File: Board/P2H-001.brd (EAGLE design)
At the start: 94.9 x 72.4 mm, 29 parts, among them IC1 74LS157N, IC2 LTC485N, IC3 74LS07N, IC4 LTC485N, IC5 TLC5941NT, IC6 TLC5941NT

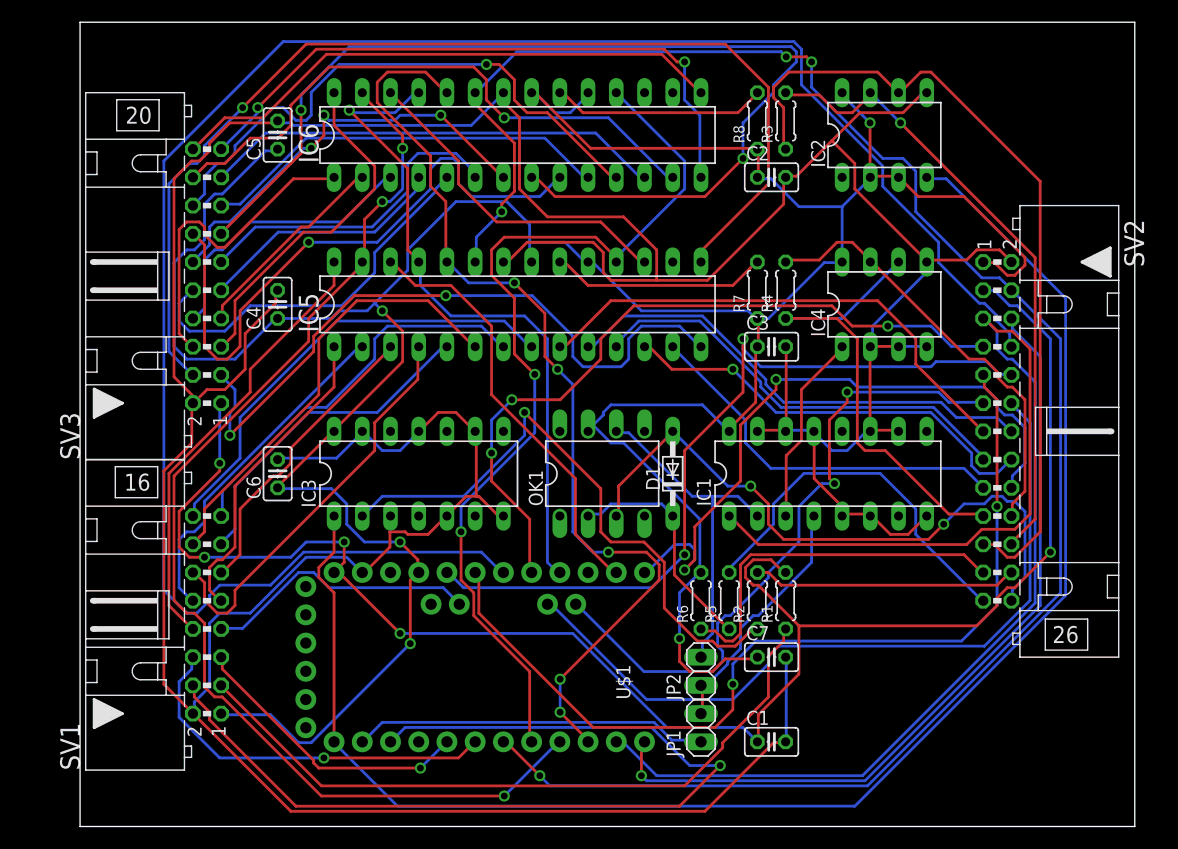
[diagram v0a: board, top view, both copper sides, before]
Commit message: square design.
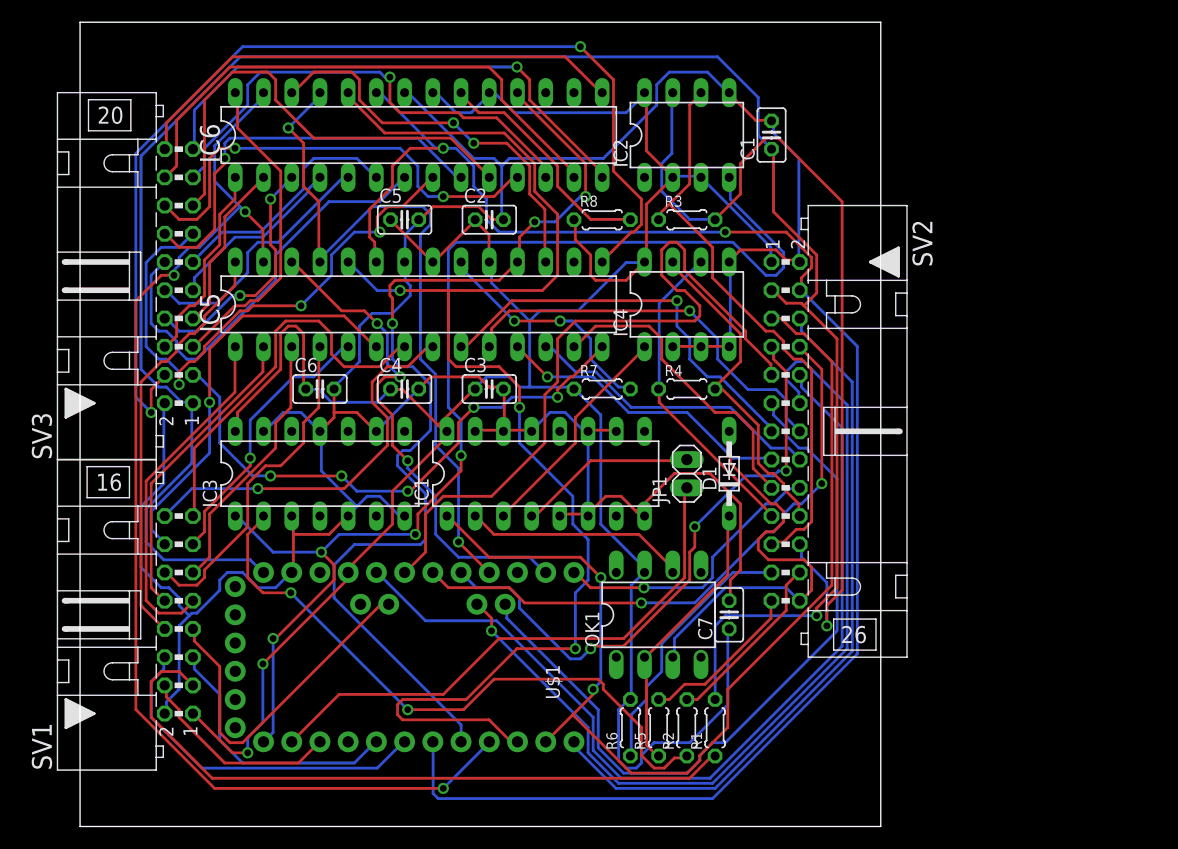
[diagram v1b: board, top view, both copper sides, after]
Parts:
- removed JP2: (no value), pinhead:1X02
- moved C1 54.6 mm to (62.2, 62.2), turned to 90 degrees
- moved C2 25.7 mm to (36.8, 54.6)
- moved C3 25.7 mm to (36.8, 39.4)
- moved IC1 25.4 mm to (41.9, 31.8)
- moved JP1 22.9 mm to (54.6, 31.8)
- moved SV2 19.0 mm to (63.5, 35.6)
- moved IC2 17.8 mm to (54.6, 62.2)
- moved IC4 17.8 mm to (54.6, 47.0)
- moved R7 16.6 mm to (47.0, 39.4), turned to 0 degrees
- moved R8 16.6 mm to (47.0, 54.6), turned to 0 degrees
- moved C4 13.7 mm to (29.2, 39.4), turned to 0 degrees
- moved C5 13.7 mm to (29.2, 54.6), turned to 0 degrees
- moved OK1 13.7 mm to (52.1, 19.1)
- moved R1 13.1 mm to (57.1, 8.89)
- moved R2 13.1 mm to (54.6, 8.89)
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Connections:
- net MIDIRX: no longer JP2.2
- net N$1: no longer JP2.1
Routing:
- net GND: track 400.2 -> 265.3 mm
- net N$8: track 170.4 -> 54.1 mm, vias 0 -> 2
- net SWRST: track 86.0 -> 18.6 mm, vias 1 -> 0
- net VCC: track 310.3 -> 252.1 mm, vias 5 -> 2
- net N$30: track 94.8 -> 51.6 mm, vias 2 -> 3
- net XLAT: track 87.3 -> 122.1 mm, vias 5 -> 3
- net N$17: track 59.0 -> 25.7 mm, vias 2 -> 1
- net TX: track 141.3 -> 108.4 mm, vias 0 -> 4
- net VDD: track 154.4 -> 182.7 mm, vias 5 -> 1
- net XBAR: track 122.7 -> 94.9 mm, vias 0 -> 2
- net TX-: track 56.9 -> 80.8 mm
- net TX+: track 74.3 -> 52.1 mm
- net N$40: track 56.7 -> 36.8 mm
- net BLANK: track 168.5 -> 149.2 mm, vias 4 -> 2
- net N$18: track 34.0 -> 14.7 mm
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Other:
- board size 94.9 x 72.4 mm -> 72.1 x 72.4 mm
